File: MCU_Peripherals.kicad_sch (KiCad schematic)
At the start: 24 parts

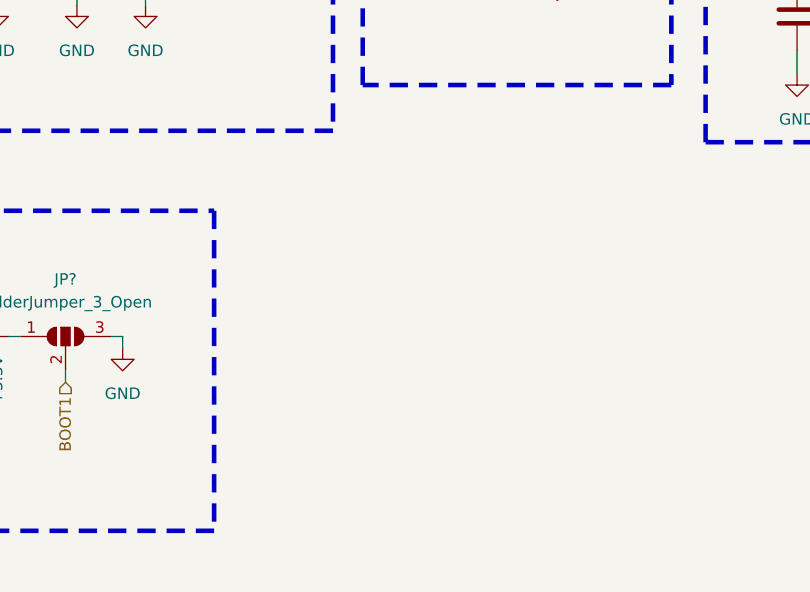
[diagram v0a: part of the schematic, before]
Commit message: Stepper Motor Control Update
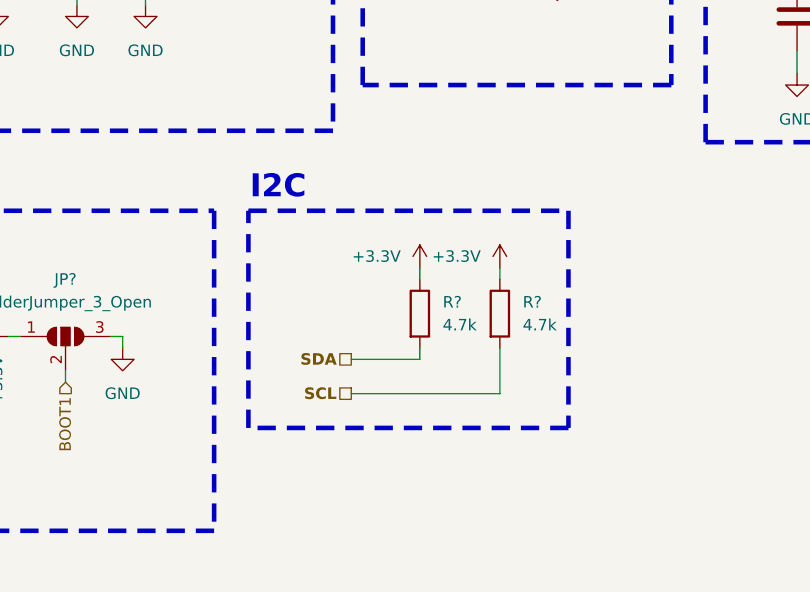
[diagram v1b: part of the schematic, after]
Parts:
- added R? (x2): 4.7k, symbol Device:R
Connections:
- net +3.3V: now also R?.1, R?.1
- new net SCL: R?.2
- new net SDA: R?.2
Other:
- note added: "I2C"

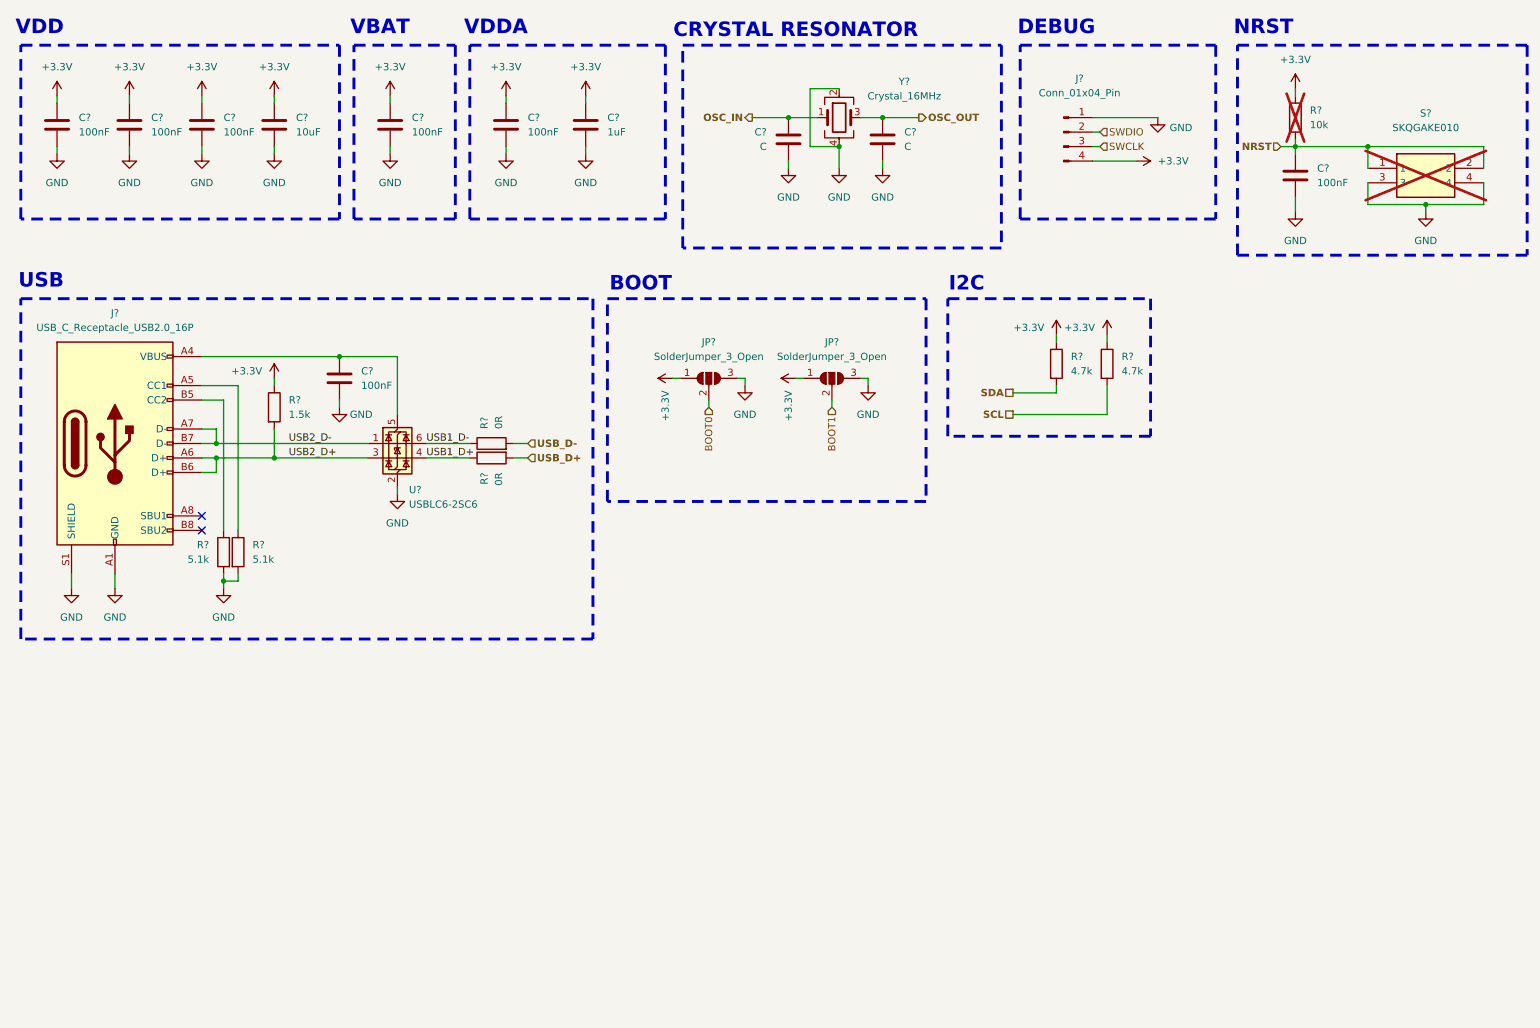
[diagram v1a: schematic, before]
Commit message: CAN & EEPROM Update
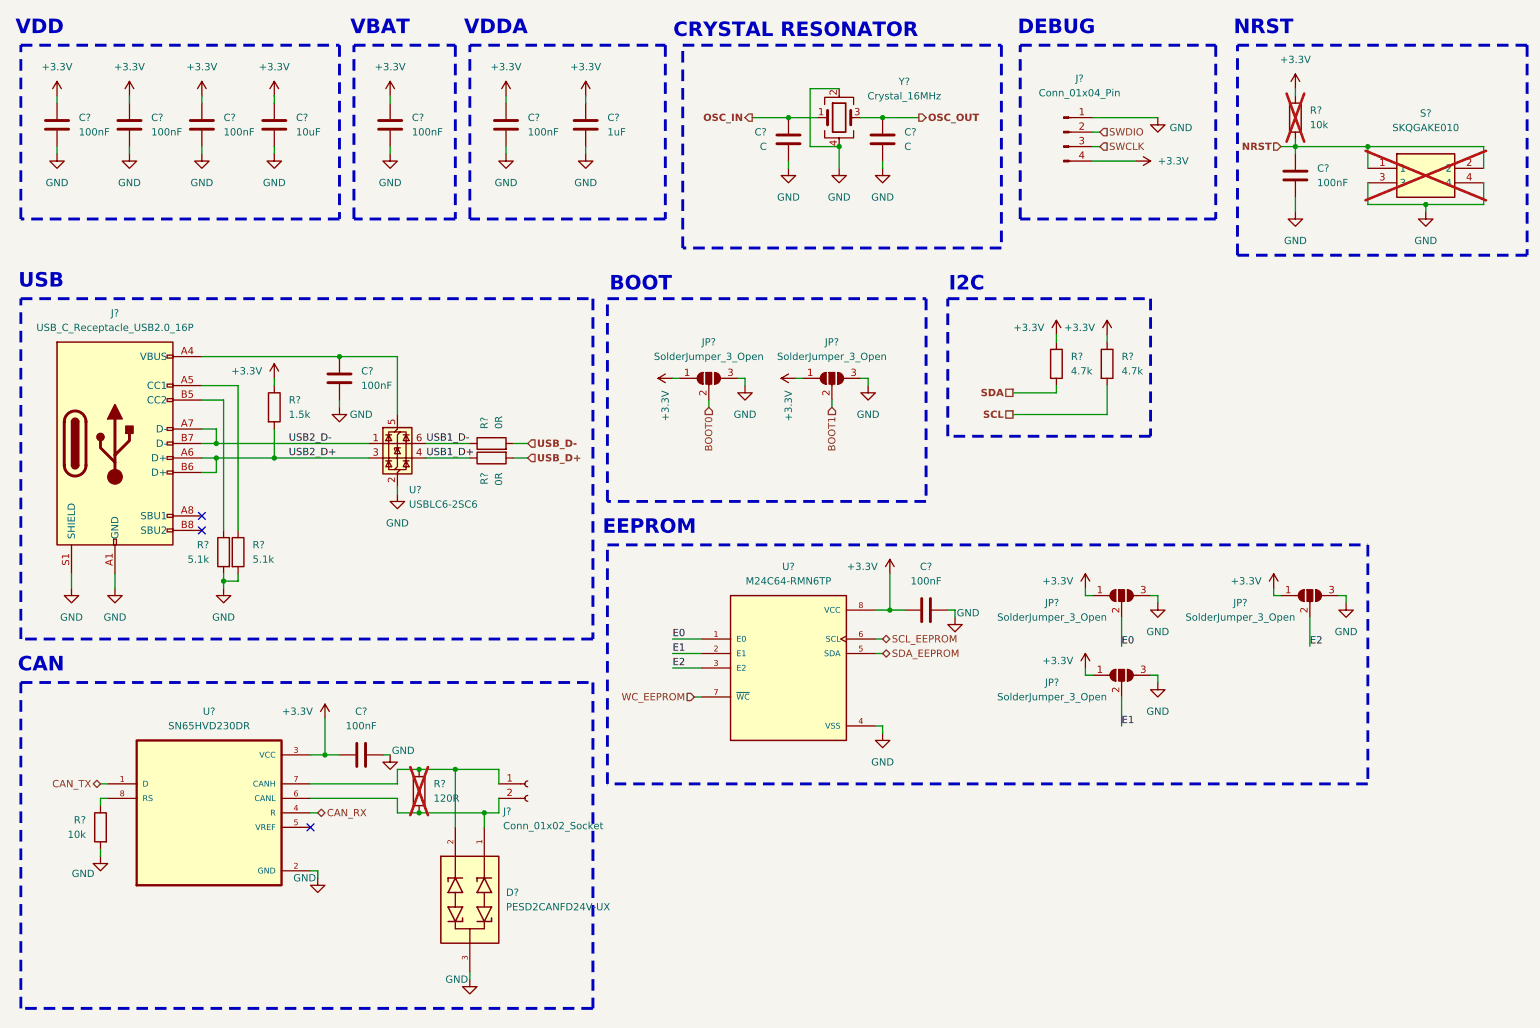
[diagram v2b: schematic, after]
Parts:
- added C? (x2): 100nF, symbol Device:C
- added D?: PESD2CANFD24V-UX, KSZ_KiCad_Footprint_Library:TVS_PESD2CANFD24V-UX, symbol KSZ_KiCad_Symbol_Library:PESD2CANFD24V-UX
- added J?: Conn_01x02_Socket, symbol Connector:Conn_01x02_Socket
- added JP? (x3): SolderJumper_3_Open, symbol Jumper:SolderJumper_3_Open
- added R?: 120R, symbol Device:R
- added R?: 10k, symbol Device:R
- added U?: SN65HVD230DR, KSZ_KiCad_Footprint_Library:SOIC127P599X175-8N, symbol KSZ_KiCad_Symbol_Library:SN65HVD230DR
- added U?: M24C64-RMN6TP, KSZ_KiCad_Footprint_Library:SOIC127P600X175-8N, symbol KSZ_KiCad_Symbol_Library:M24C64-RMN6TP
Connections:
- net +3.3V: now also C?.1, C?.1, JP?.1 (A), JP?.1 (A), JP?.1 (A), U?.3 (VCC), U?.8 (VCC)
- net GND: now also C?.2, C?.2, D?.3, JP?.3 (B), JP?.3 (B), JP?.3 (B), R?.2, U?.2 (GND), U?.4 (VSS)
- new net: D?.1, J?.2 (Pin_2), R?.2, U?.6 (CANL)
- new net: D?.2, J?.1 (Pin_1), R?.1, U?.7 (CANH)
- new net: R?.1, U?.8 (RS)
- new net CAN_RX: U?.4 (R)
- new net CAN_TX: U?.1 (D)
- new net E0: JP?.2 (C), U?.1 (E0)
- new net E1: JP?.2 (C), U?.2 (E1)
- new net E2: JP?.2 (C), U?.3 (E2)
- new net SCL_EEPROM: U?.6 (SCL)
- new net SDA_EEPROM: U?.5 (SDA)
- new net WC_EEPROM: U?.7 (~{WC})
- no-connect marks 2 -> 3
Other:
- note added: "CAN"
- note added: "EEPROM"

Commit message: LEDs, Button & Small fixes
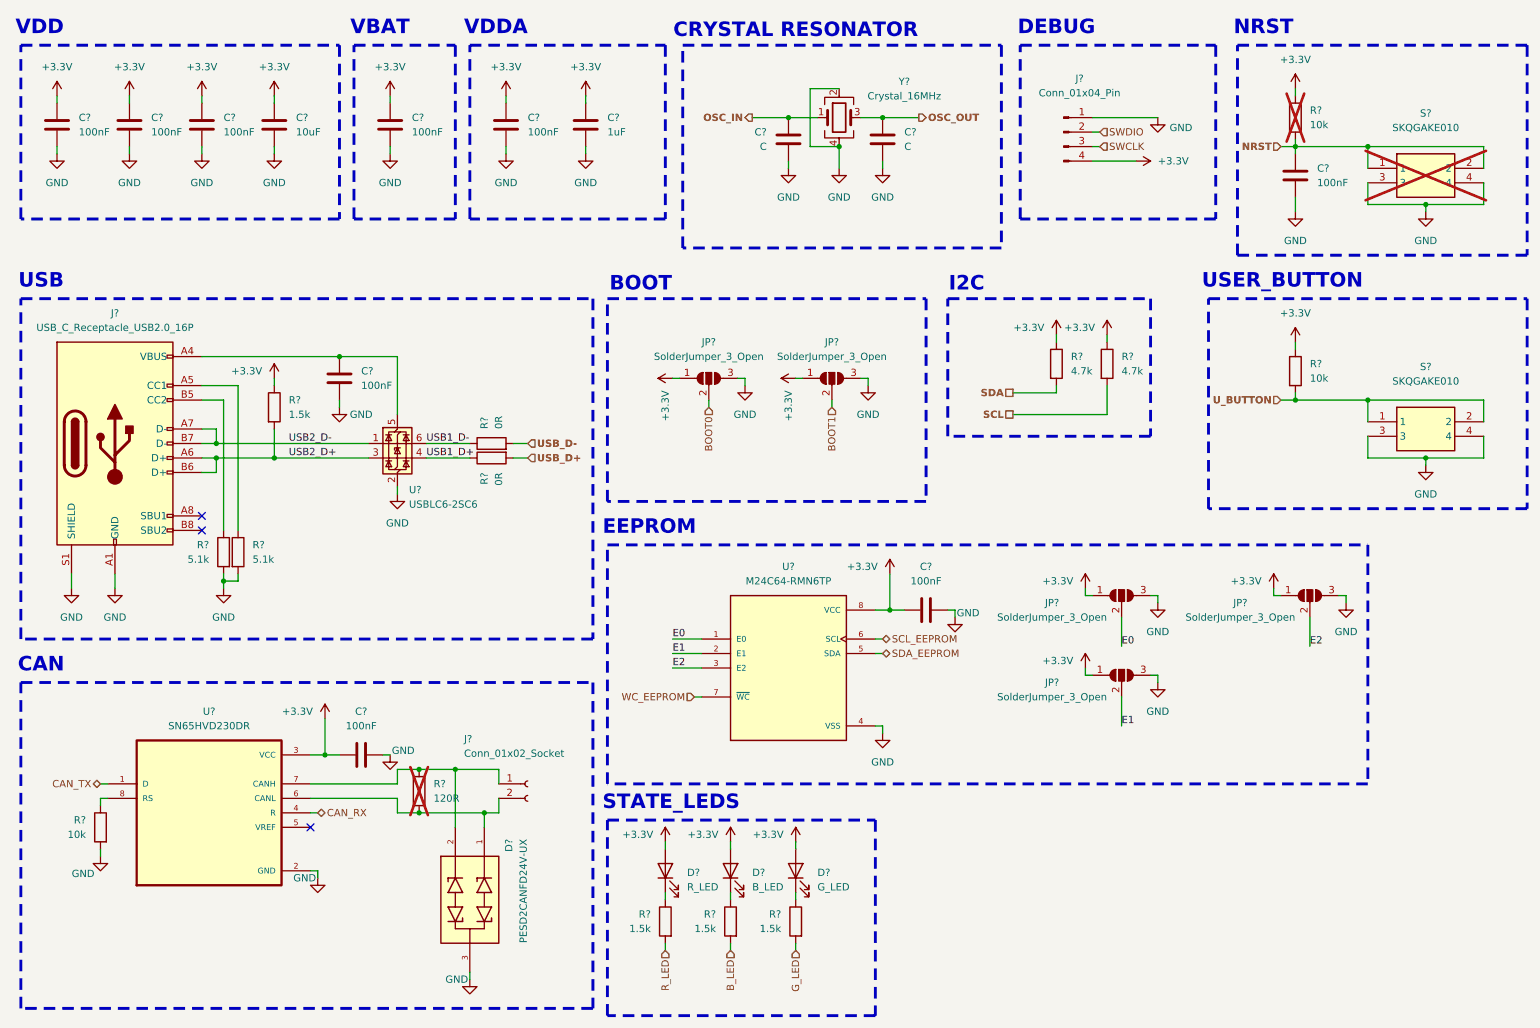
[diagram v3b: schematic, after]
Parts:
- added D?: R_LED, symbol Device:LED
- added D?: B_LED, symbol Device:LED
- added D?: G_LED, symbol Device:LED
- added R? (x3): 1.5k, symbol Device:R
- added R?: 10k, symbol Device:R
- added S?: SKQGAKE010, KSZ_KiCad_Footprint_Library:SKQGAKE010, symbol KSZ_KiCad_Symbol_Library:SKQGAKE010
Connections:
- net +3.3V: now also D?.2 (A), D?.2 (A), D?.2 (A), R?.1
- net GND: now also S?.3, S?.4
- new net: D?.1 (K), R?.1 (x3)
- new net B_LED: R?.2
- new net G_LED: R?.2
- new net R_LED: R?.2
- new net U_BUTTON: R?.2, S?.1, S?.2
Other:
- note added: "STATE_LEDS"
- note added: "USER_BUTTON"
